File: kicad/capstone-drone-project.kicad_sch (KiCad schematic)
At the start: 35 parts, among them J1 CU01SAV0S00, Q1 PMOS, Q2 PMOS, Q3 NMOS, U1 ESP32-S3, Y1 ECS-400-10-37B2-CKY-TR

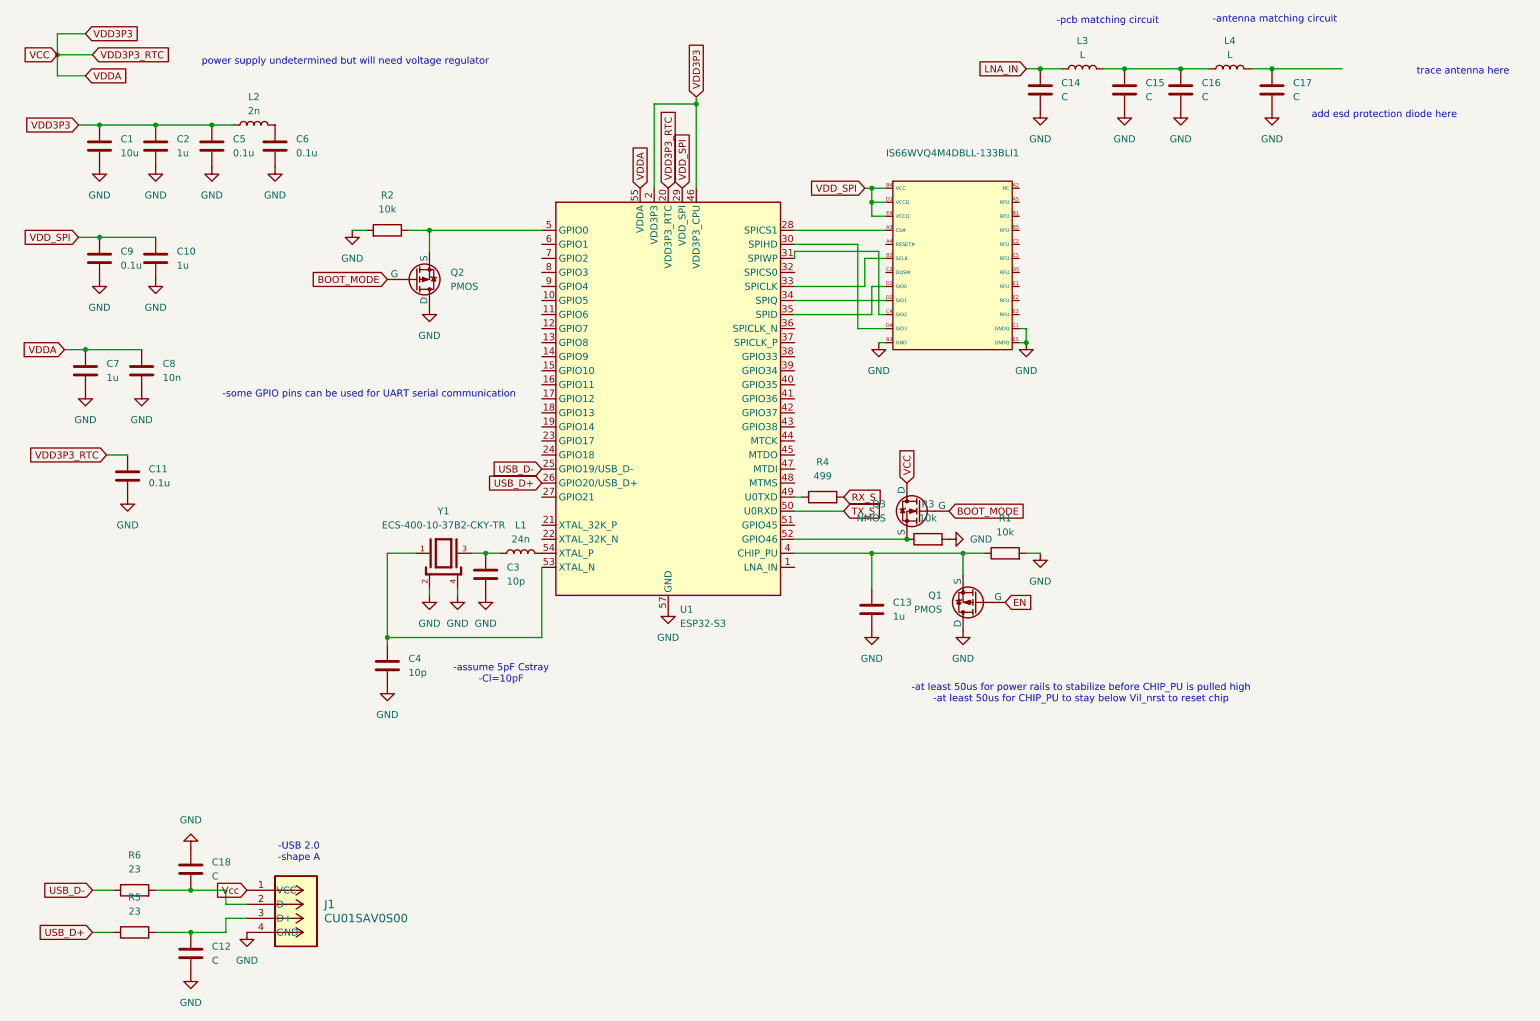
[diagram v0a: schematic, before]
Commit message: draft
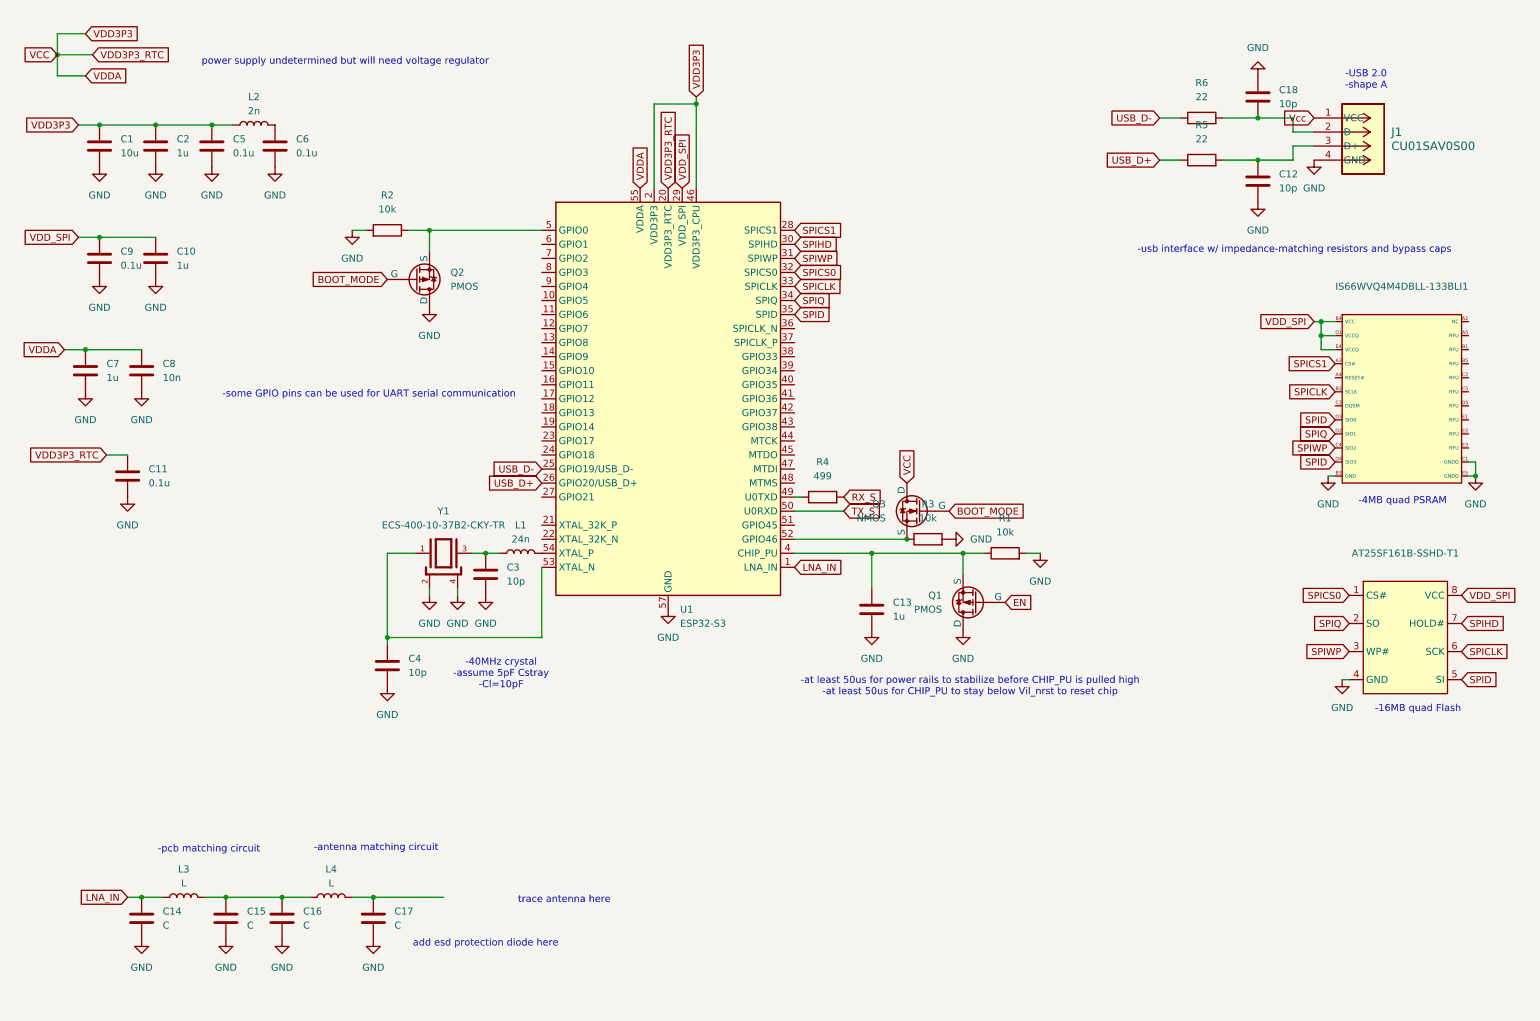
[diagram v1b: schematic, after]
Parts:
- added AT25SF161B-SSHD-T1: ~, symbol capstone-drone-project-custom-symbols:AT25SF161B-SSHD-T
- C12, C18: value C -> 10p
- R5, R6: value 23 -> 22
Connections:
- net GND: now also AT25SF161B-SSHD-T1.4 (GND)
- net LNA_IN: now also U1.1 (LNA_IN)
- net VDD_SPI: now also AT25SF161B-SSHD-T1.8 (VCC)
- net SPICS1: now reaches IS66WVQ4M4DBLL-133BLI1.A3 (CS#), U1.28 (SPICS1)
- net SPID: now reaches IS66WVQ4M4DBLL-133BLI1.D4 (SIO3)
- net SPID: now also IS66WVQ4M4DBLL-133BLI1.D3 (SIO0), U1.35 (SPID), AT25SF161B-SSHD-T1.5 (SI); no longer U1.30 (SPIHD)
- net SPIWP: now reaches IS66WVQ4M4DBLL-133BLI1.C4 (SIO2), U1.31 (SPIWP)
- net SPIWP: now also AT25SF161B-SSHD-T1.3 (WP#)
- net SPICS0: now reaches U1.32 (SPICS0)
- net SPICS0: now also AT25SF161B-SSHD-T1.1 (CS#)
- net SPICLK: now reaches IS66WVQ4M4DBLL-133BLI1.B2 (SCLK), U1.33 (SPICLK)
- net SPICLK: now also AT25SF161B-SSHD-T1.6 (SCK)
- net SPIQ: now reaches IS66WVQ4M4DBLL-133BLI1.D2 (SIO1), U1.34 (SPIQ)
- net SPIQ: now also AT25SF161B-SSHD-T1.2 (SO)
- new net SPIHD: AT25SF161B-SSHD-T1.7 (HOLD#), U1.30 (SPIHD)
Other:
- note added: "-16MB quad Flash"
- note added: "-40MHz crystal -assume 5pF Cstray -Cl=10pF"
- note added: "-4MB quad PSRAM"
- note added: "-usb interface w/ impedance-matching resistors and bypass caps"
- note removed: "-assume 5pF Cstray -Cl=10pF"
- moved on the sheet: C12, C14, C15, C16, C17, C18, IS66WVQ4M4DBLL-133BLI1, J1, L3, L4, R5, R6
